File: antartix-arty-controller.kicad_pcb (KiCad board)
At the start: 4 copper layers, 68.5 x 40 mm, 103 parts, among them IC1 FT2232D, J1 QTE-020-04-L-D-A, J2 614004185023, J3 614004185023, J4 614004185023, J5 WE_629105150521, U1 PCT2075GVX, U2 PAC1934T-I_JQ, U3 USB2514B-I_M2, U4 TPS2024DR, U5 TPS2024DR, U6 TPS2024DR, U7 TPS2051BDBVR, Y1 7C-24.000MBB-T, Y2 MQ-6.000-12-30_30_

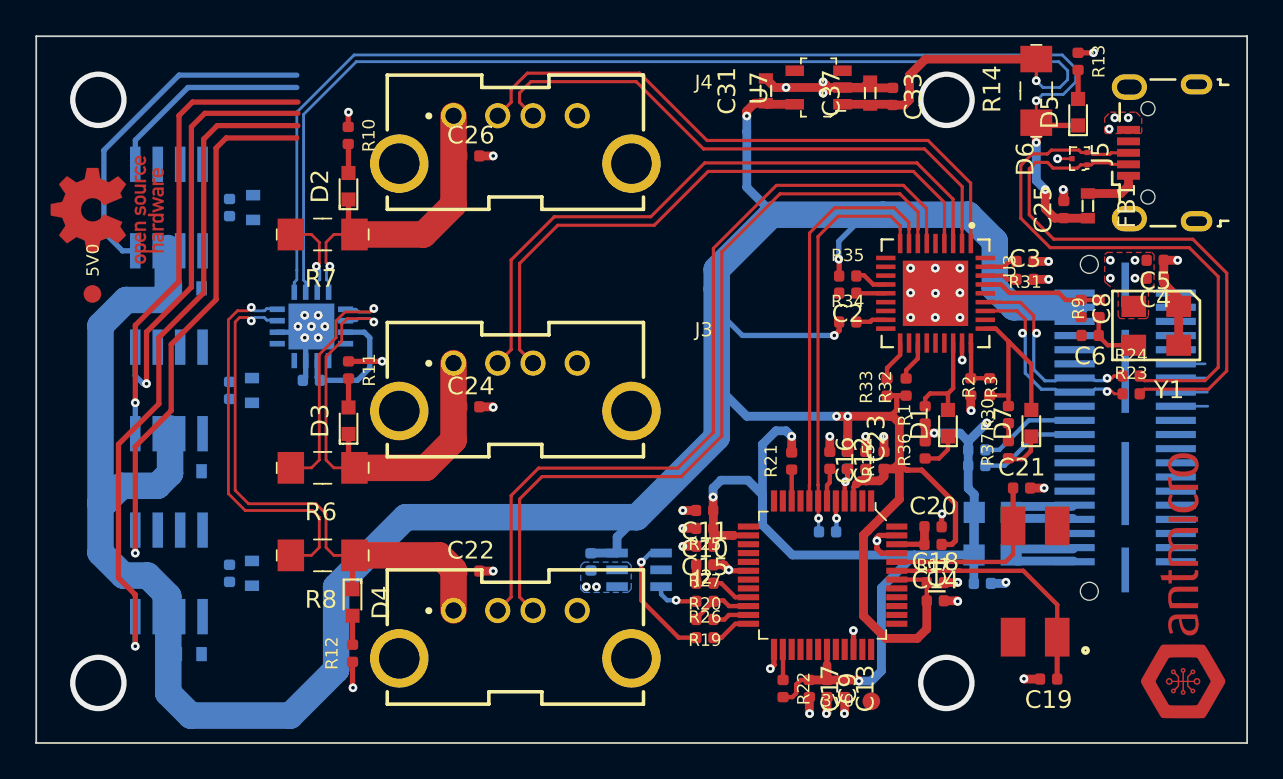
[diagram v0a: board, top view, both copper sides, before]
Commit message: Board routed
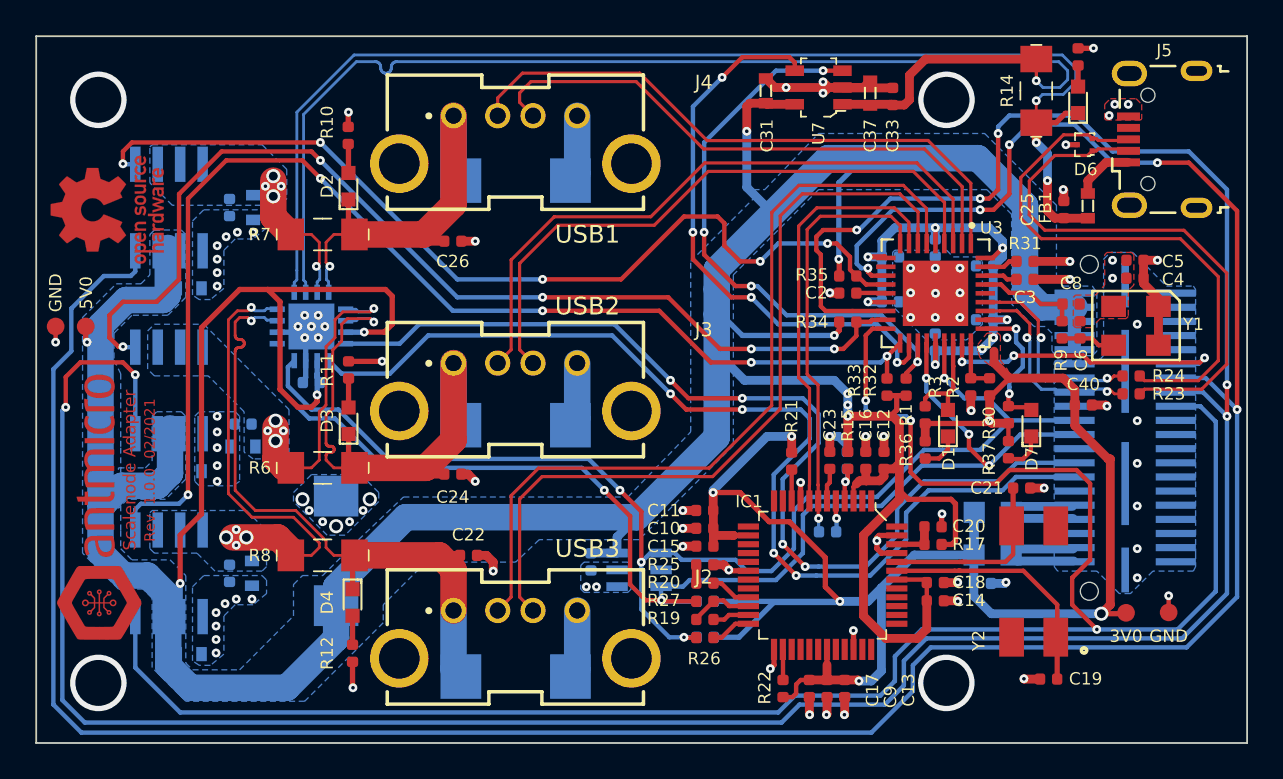
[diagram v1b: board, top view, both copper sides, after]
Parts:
- added C40: C_1u_0402, antmicro-footprints:0402-cap, F.Cu at (165.8, 78.7)
- added C41: C_100n_0402, antartix-arty-controller-footprints:0402-cap, B.Cu at (157.5, 69.8)
- added C42: C_100n_0402, antartix-arty-controller-footprints:0402-cap, B.Cu at (160.2, 70.9)
- added C43: C_100n_0402, antartix-arty-controller-footprints:0402-cap, B.Cu at (154.9, 70.3)
- added C44: C_100n_0402, antartix-arty-controller-footprints:0402-cap, B.Cu at (160.2, 73.9)
- added C45: C_100n_0402, antartix-arty-controller-footprints:0402-cap, B.Cu at (154.9, 72.9)
- added C46: C_100n_0402, antartix-arty-controller-footprints:0402-cap, B.Cu at (157.5, 75.2)
- added C47: C_330u_KEMET_D, antmicro-footprints:KEMET_D, B.Cu at (133.7, 66.0)
- added C48: C_330u_KEMET_D, antmicro-footprints:KEMET_D, B.Cu at (133.7, 79.9)
- added C49: C_330u_KEMET_D, antmicro-footprints:KEMET_D, B.Cu at (133.7, 94.1)
- added C50: C_680u_KEMET_D, antmicro-footprints:KEMET_D, B.Cu at (123.5, 87.0)
- added GND: TP_SMD1MM, antartix-arty-controller-footprints:Testpoint_smd_1mm, F.Cu at (107.6, 74.3)
- added GND: TP_SMD1MM, antartix-arty-controller-footprints:Testpoint_smd_1mm, F.Cu at (170.7, 90.4)
- moved N1 61.5 mm to (110.2, 84.1)
- moved R4 18.7 mm to (144.4, 91.9), turned to 0 degrees
- moved R5 17.2 mm to (144.4, 89.8), turned to 180 degrees
- moved 3V0 15.3 mm to (168.2, 90.5)
- moved C26 4.93 mm to (130.1, 69.5)
- moved C24 3.94 mm to (130.1, 82.6)
- moved C36 3.22 mm to (118.3, 81.1), turned to 0 degrees
- moved R9 2.42 mm to (164.6, 74.5)
- moved C32 2.05 mm to (118.3, 79.8), turned to 0 degrees
- moved 5V0 1.88 mm to (109.3, 74.3)
- moved C4 1.14 mm to (168.8, 71.6)
- moved C5 1.14 mm to (168.8, 70.5)
- moved Y1 1.14 mm to (169.1, 74.0)
- moved C22 0.90 mm to (131.0, 87.2)
- moved D6 0.84 mm to (165.9, 64.0)
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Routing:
- net /USB1_EN: track 21.2 -> 157.3 mm, vias 0 -> 5
- net /USB2_EN: track 27.9 -> 160.6 mm, vias 1 -> 7
- net VCC3V3: track 69.9 -> 172.2 mm, vias 6 -> 15
- net /USB3_EN: track 40.2 -> 112.5 mm, vias 1 -> 3
- net SDA0: track 8.37 -> 73.2 mm, vias 1 -> 5
- net /SLOW_~ALERT: track 0.00 -> 59.6 mm, vias 0 -> 4
- net SCL0: track 13.2 -> 71.2 mm, vias 1 -> 4
- net /~PWRDN: track 0.00 -> 57.9 mm, vias 0 -> 4
- net VCC5V0: track 201.7 -> 251.2 mm, vias 5 -> 10
- net /OC_N1: track 13.6 -> 53.1 mm, vias 0 -> 5
- net /OC_N3: track 33.2 -> 68.9 mm, vias 1 -> 5
- net /OC_N2: track 26.1 -> 59.3 mm, vias 1 -> 5
- net /USB4_EN: track 0.00 -> 32.3 mm, vias 0 -> 4
- net /OC_N4: track 2.28 -> 33.1 mm, vias 0 -> 4
- net GND: track 46.1 -> 66.8 mm, vias 59 -> 95
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- added copper zone on B.Cu, net VBUS1_S
- added copper zone on B.Cu, net VBUS2_S
- added copper zone on B.Cu, net VBUS3_S
- added copper zone on F.Cu, net VCC3V3
- added copper zone on B.Cu, net VCC5V0
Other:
- board text added: "Rev. 1.0.0 02/2021"
- board text added: "Scalenode Adapter"
- board text added: "USB1"
- board text added: "USB2"
- board text added: "USB3"
